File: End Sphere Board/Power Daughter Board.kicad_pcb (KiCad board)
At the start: 2 copper layers, 35.4 x 38.9 mm, 29 parts, among them J1 End_Sphere_Conn, J2 Jack-DC, SW1 MHPS2283, U1 MCP73833T

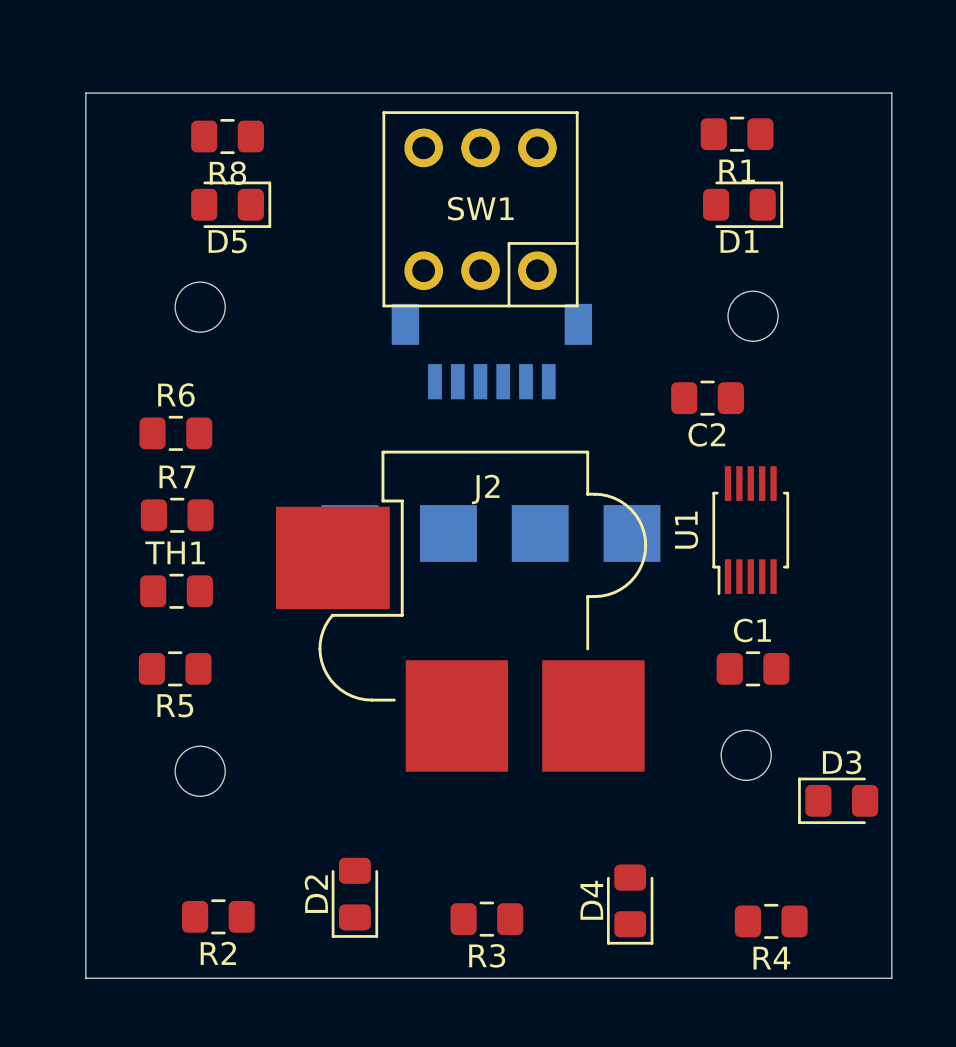
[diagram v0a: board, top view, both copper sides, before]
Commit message: PCB preliminary version
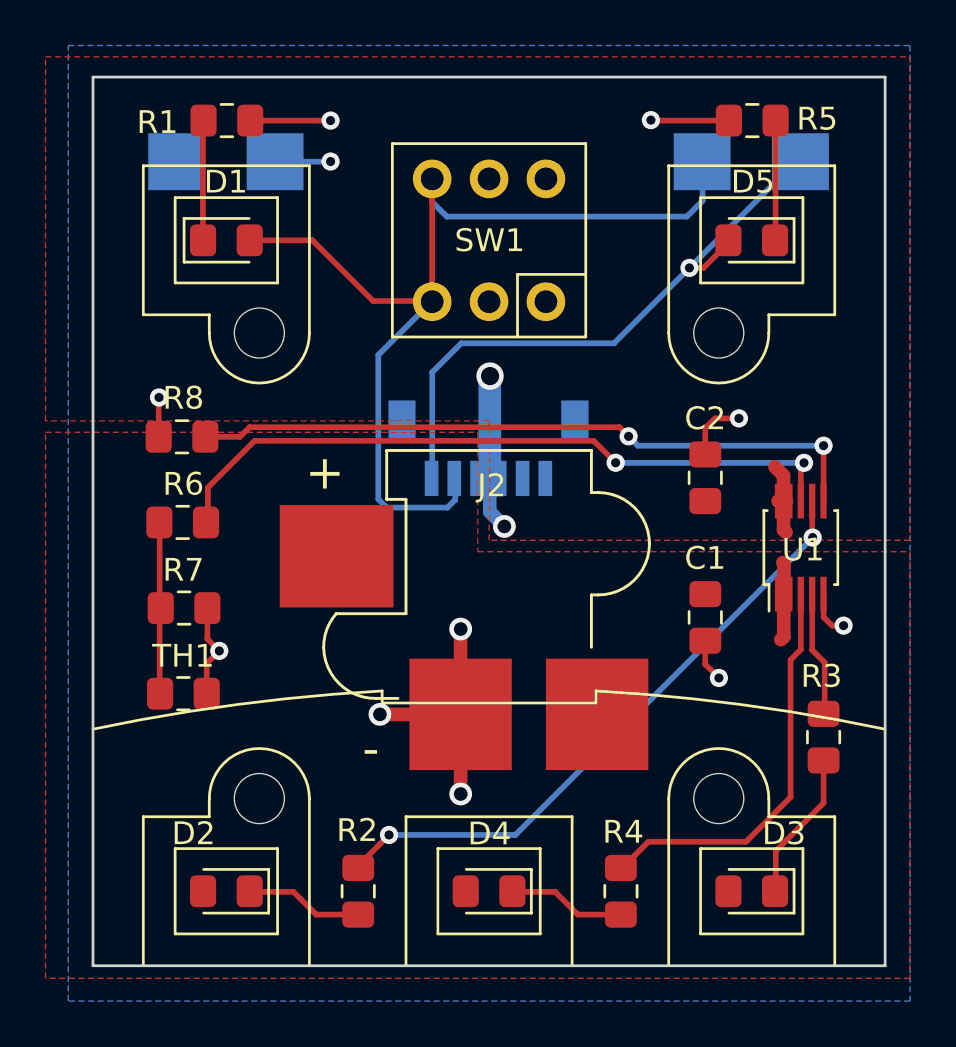
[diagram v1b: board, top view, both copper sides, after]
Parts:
- moved D5 23.1 mm to (157.0, 95.6)
- moved R5 23.1 mm to (157.1, 90.3)
- moved D1 22.6 mm to (134.0, 95.6), turned to 0 degrees
- moved R1 22.4 mm to (134.0, 90.3), turned to 0 degrees
- moved TP3 18.0 mm to (136.1, 92.1)
- moved TP4 18.0 mm to (131.8, 92.1)
- moved TP1 17.9 mm to (159.2, 92.1)
- moved TP2 17.8 mm to (154.9, 92.1)
- moved R3 16.8 mm to (160.2, 117.4), turned to 270 degrees
- moved R8 10.2 mm to (132.0, 104.2)
- moved WA1 9.39 mm to (144.7, 137.3)
- moved R4 6.74 mm to (151.3, 124.2), turned to 270 degrees
- moved R2 6.25 mm to (139.7, 124.2), turned to 270 degrees
- moved D4 6.22 mm to (145.5, 124.2), turned to 180 degrees
- moved D2 5.65 mm to (134.0, 124.2), turned to 180 degrees
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- renumbered R8 to R5, R5 to R8
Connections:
- net Net-(D1-Pad1) renamed /ON
- net Net-(D5-Pad1) renamed /RDYIND
- D1 pad 2: /BATT+ -> /SWITCH
- D5 pad 2: /BATT+ -> /READY
- R1 pad 2: /SWITCH -> GND
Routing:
- net /SWITCH: track 0.00 -> 44.0 mm
- net /THRMIC: track 0.00 -> 30.7 mm, vias 0 -> 2
- net GND: track 0.00 -> 30.6 mm, vias 0 -> 10
- net /PROG: track 0.00 -> 30.1 mm, vias 0 -> 2
- net /PG: track 0.00 -> 27.5 mm, vias 0 -> 2
- net /READY: track 0.00 -> 26.6 mm, vias 0 -> 1
- net /ST1: track 0.00 -> 17.9 mm
- net /BATT+: track 0.00 -> 13.5 mm, vias 0 -> 3
- net /THRM: track 0.00 -> 7.75 mm
- net Net-(D3-Pad1): track 0.00 -> 6.59 mm
- net /ST2: track 0.00 -> 5.61 mm
- net /ON: track 0.00 -> 5.34 mm
- net /RDYIND: track 0.00 -> 5.32 mm
- net Net-(D2-Pad1): track 0.00 -> 5.16 mm
- net Net-(D4-Pad1): track 0.00 -> 5.11 mm
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- added copper zone on F.Cu, net /BATT+
- added copper zone on F.Cu, net /PWRIN
- added copper zone on B.Cu, net GND
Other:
- board size 35.4 x 38.9 mm -> 34.8 x 39.1 mm
- net class Power added: clearance 0.2, trace_width 0.6, via_dia 1, via_drill 0.6
- board text added: "+"
- board text added: "-"
- board text added: "B+"
- board text added: "G"
- board text added: "RDY"
- board text added: "SW"
